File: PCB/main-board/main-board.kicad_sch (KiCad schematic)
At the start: 42 parts, among them CN2 XT30APB, J2 Motor (JST-PH 2P), U1 ESP32-S3-SuperMini, U2 DRV8876RGTR, U3 MLX90393SLW-ABA-011-RE, U4 AP63205WU-7, U5 SN65HVD230

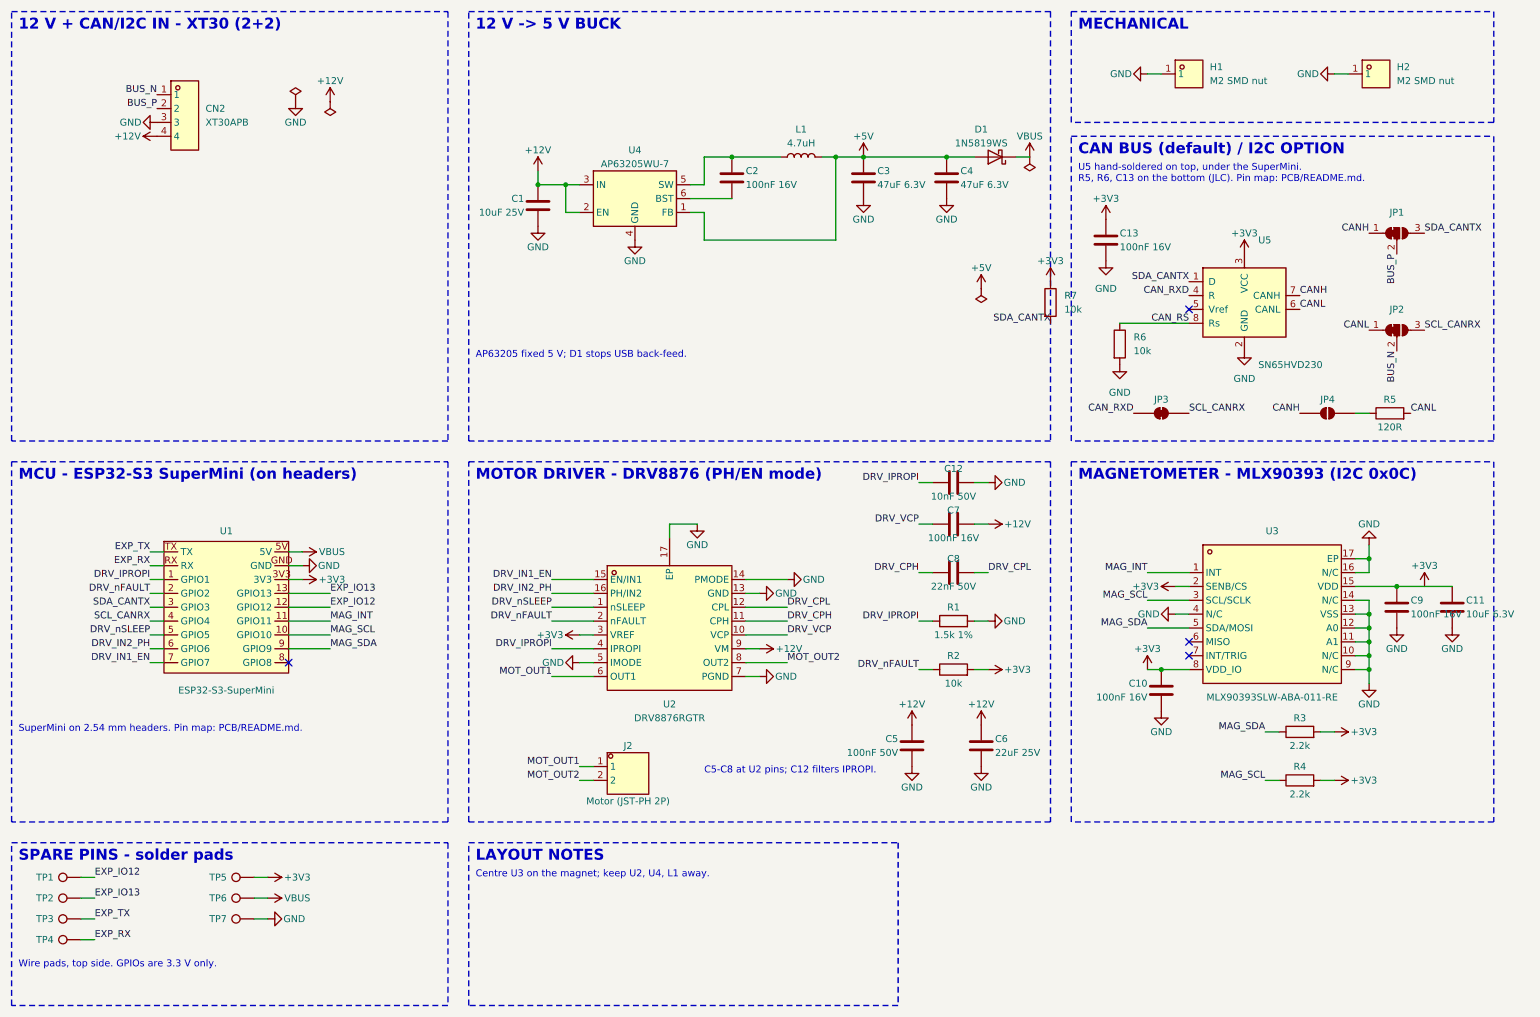
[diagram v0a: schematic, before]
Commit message: new schematic
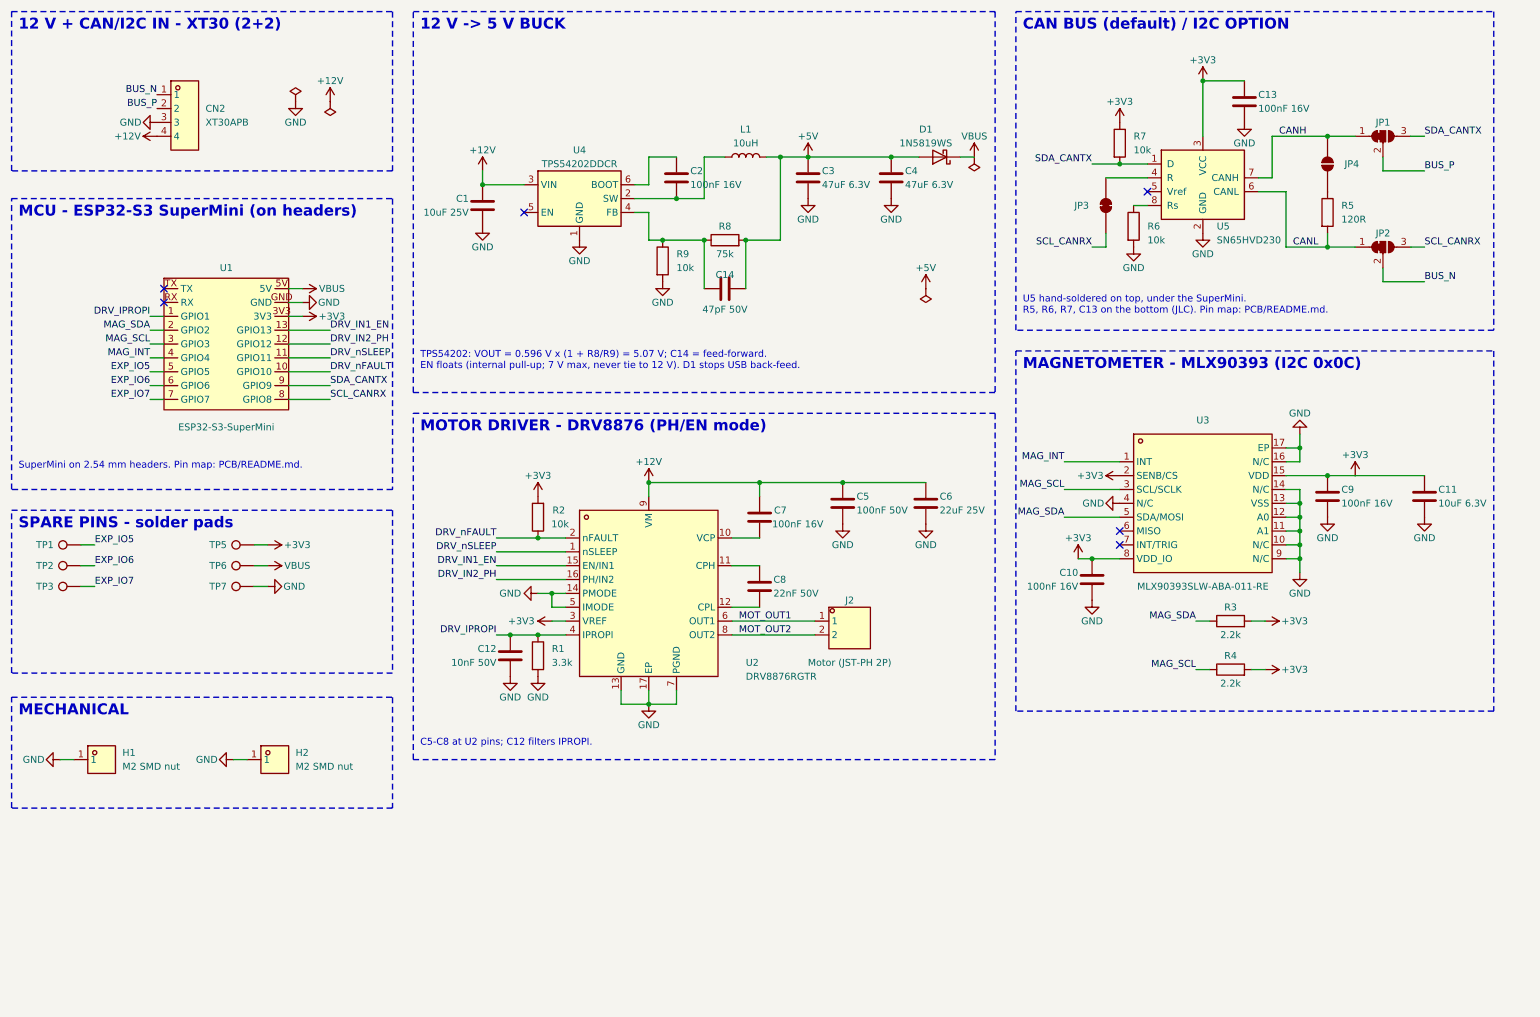
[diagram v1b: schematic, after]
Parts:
- removed TP4: Pad, TestPoint:TestPoint_Pad_D1.5mm, symbol Connector:TestPoint
- added C14: 47pF 50V, Capacitor_SMD:C_0402_1005Metric, symbol Device:C
- added R8: 75k, Resistor_SMD:R_0402_1005Metric, symbol Device:R
- added R9: 10k, Resistor_SMD:R_0402_1005Metric, symbol Device:R
- L1: value 4.7uH -> 10uH; LCSC Part C5832374 -> C5832376; MPN FTC252012S4R7MBCA -> FTC252012S100MBCA
- R1: value 1.5k 1% -> 3.3k; footprint Resistor_SMD:R_0402_1005Metric -> Resistor_SMD:R_0805_2012Metric_Pad1.20x1.40mm_HandSolder; LCSC Part C25867 -> C26010; MPN 0402WGF1501TCE -> 0805W8F3301T5E
- U4: value AP63205WU-7 -> TPS54202DDCR; symbol Regulator_Switching:AP63205WU -> Regulator_Switching:TPS54202DDC; LCSC Part C2071056 -> C191884; MPN AP63205WU-7 -> TPS54202DDCR; Manufacturer Diodes Incorporated -> Texas Instruments
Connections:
- net +12V: no longer U4.2 (EN)
- net +5V: now also C14.2, R8.2; no longer U4.1 (FB)
- net DRV_IN1_EN: now also U1.13 (GPIO13); no longer U1.7 (GPIO7)
- net DRV_IN2_PH: now also U1.12 (GPIO12); no longer U1.6 (GPIO6)
- net DRV_nFAULT: now also U1.10 (GPIO10); no longer U1.2 (GPIO2)
- net DRV_nSLEEP: now also U1.11 (GPIO11); no longer U1.5 (GPIO5)
- net GND: now also U4.1 (GND), R9.2; no longer U4.4 (GND)
- net MAG_INT: now also U1.4 (GPIO4); no longer U1.11 (GPIO11)
- net MAG_SCL: now also U1.3 (GPIO3); no longer U1.10 (GPIO10)
- net MAG_SDA: now also U1.2 (GPIO2); no longer U1.9 (GPIO9)
- net SCL_CANRX: now also U1.8 (GPIO8); no longer U1.4 (GPIO4)
- net SDA_CANTX: now also U1.9 (GPIO9); no longer U1.3 (GPIO3)
- net at U4.6 (BOOT): now also C2.1; no longer C2.2
- net CAN_RS: no longer names the net of R6.1, U5.8 (Rs)
- net CAN_RXD: no longer names the net of JP3.1 (A), U5.4 (R)
- net DRV_CPH: no longer names the net of C8.1, U2.11 (CPH)
- net DRV_CPL: no longer names the net of C8.2, U2.12 (CPL)
- net DRV_VCP: no longer names the net of C7.1, U2.10 (VCP)
- net EXP_IO12 renamed EXP_IO5
- net EXP_IO5: now also U1.5 (GPIO5); no longer U1.12 (GPIO12)
- net EXP_IO13 renamed EXP_IO6
- net EXP_IO6: now also U1.6 (GPIO6); no longer U1.13 (GPIO13)
- net EXP_RX: no longer names the net of U1.RX
- net EXP_TX: no longer names the net of U1.TX
- net EXP_TX: no longer TP3.1
- new net: C14.1, R8.1, R9.1, U4.4 (FB)
- new net: C2.2, L1.1, U4.2 (SW)
- new net EXP_IO7: TP3.1, U1.7 (GPIO7)
- now unconnected: U4.5 (SW)
- no-connect marks 4 -> 6
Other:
- note added: "TPS54202: VOUT = 0.596 V x (1 + R8/R9) = 5.07 V; C14 = feed-forward. EN floats (internal pull-up; 7 V max, never tie to 12 V). D1 stops USB back-feed."
- note added: "U5 hand-soldered on top, under the SuperMini. R5, R6, R7, C13 on the bottom (JLC). Pin map: PCB/README.md."
- note removed: "AP63205 fixed 5 V; D1 stops USB back-feed."
- note removed: "Centre U3 on the magnet; keep U2, U4, L1 away."
- note removed: "LAYOUT NOTES"
- note removed: "U5 hand-soldered on top, under the SuperMini. R5, R6, C13 on the bottom (JLC). Pin map: PCB/README.md."
- note removed: "Wire pads, top side. GPIOs are 3.3 V only."
- moved on the sheet: C1, C10, C11, C12, C13, C2, C3, C4, C5, C6, C7, C8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
